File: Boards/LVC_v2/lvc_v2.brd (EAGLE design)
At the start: 17 parts, among them U1 LMR16020

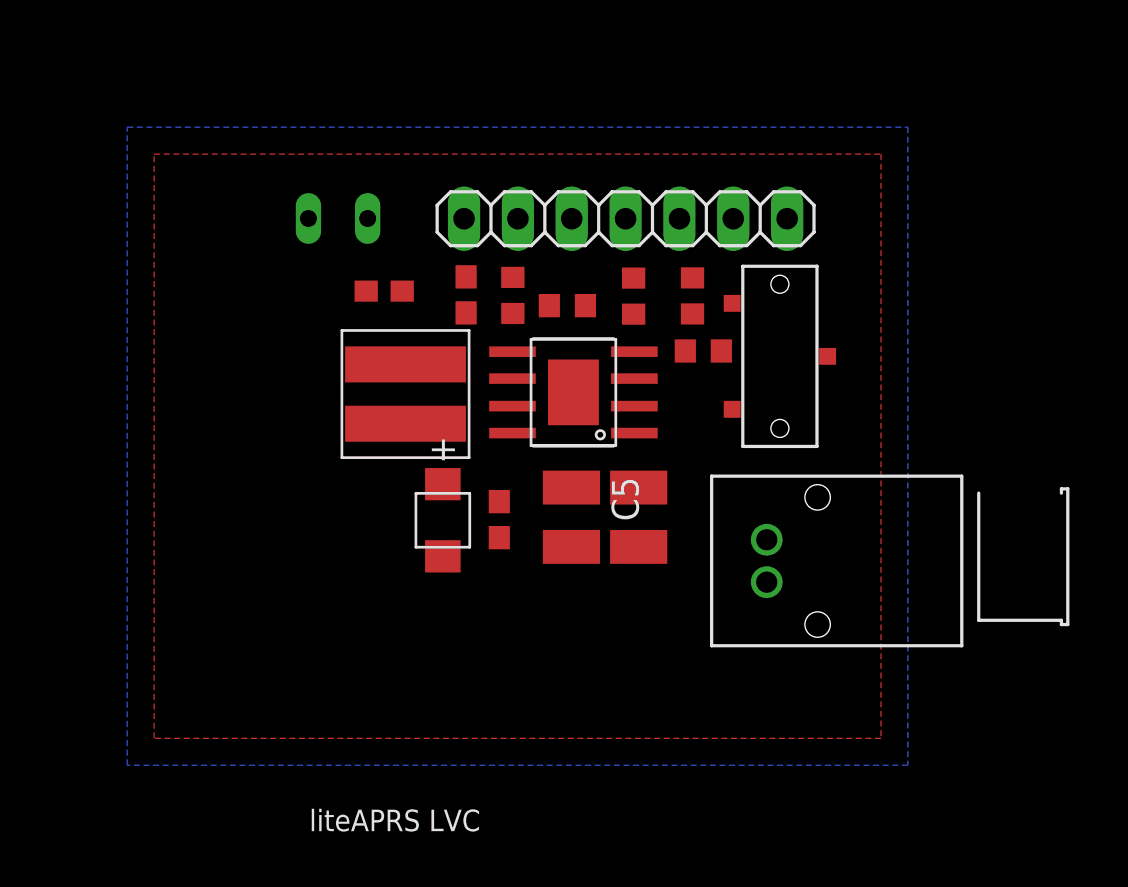
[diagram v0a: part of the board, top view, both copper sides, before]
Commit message: routed lightAPRS LVC
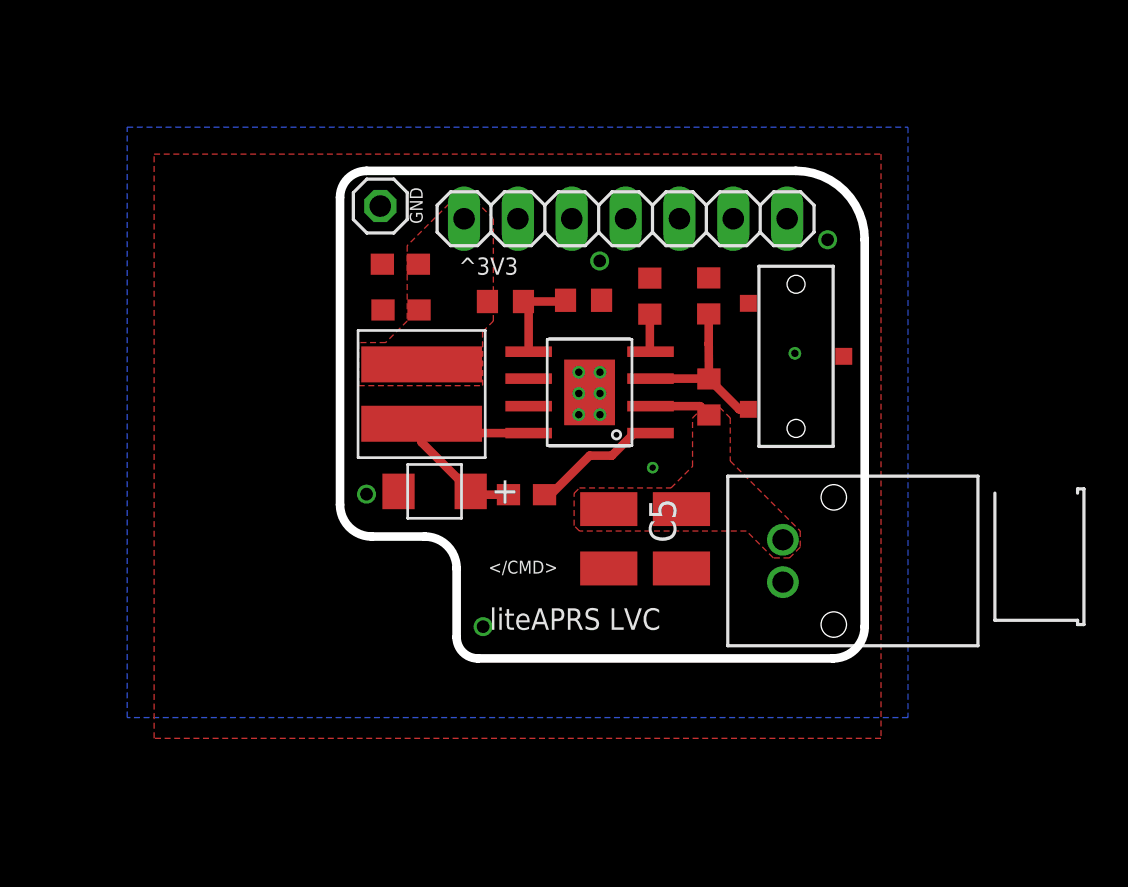
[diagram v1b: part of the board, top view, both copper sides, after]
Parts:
- removed U$2: LITEAPRS, NR_connectors:LITEAPRS
- added JP3: (no value), pinhead:1X01
- moved C4 3.15 mm to (10.4, 26.9), turned to 180 degrees
- moved C3 2.26 mm to (23.6, 16.1)
- moved R21 2.18 mm to (24.9, 22.8), turned to 270 degrees
- moved C5 2.03 mm to (20.2, 16.1)
- moved C2 1.74 mm to (16.3, 18.2), turned to 0 degrees
- moved C11 1.48 mm to (10.3, 29.1)
- moved D3 1.42 mm to (12.0, 18.4), turned to 0 degrees
- moved R19 0.80 mm to (19.0, 27.4)
- moved L1 0.76 mm to (11.4, 23.0)
- moved R17 0.76 mm to (22.1, 27.6)
- moved R20 0.76 mm to (24.9, 27.6)
- moved U$1 0.76 mm to (37.6, 19.1)
- moved U$3 0.76 mm to (30.8, 29.0)
- moved U1 0.76 mm to (19.3, 23.1)
- moved R18 0.45 mm to (15.3, 27.3), turned to 180 degrees
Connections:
- net GND: now also JP3.1; no longer U$2.P$2
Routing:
- net SW: track 0.00 -> 11.2 mm
- net N$7: track 0.00 -> 8.28 mm
- net N$31: track 0.00 -> 6.20 mm
- net FB: track 0.00 -> 4.47 mm
- net IN1: track 0.00 -> 2.93 mm
- net N$29: track 0.00 -> 1.78 mm
- added copper zone on layer 1, net +3V3
- added copper zone on layer 1, net IN1
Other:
- board outline added: 24.8 x 23 mm
- board text added: "</CMD>"
- board text added: "GND"
- board text added: "^3V3"
